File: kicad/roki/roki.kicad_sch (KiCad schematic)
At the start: 130 parts, among them SW1 RotaryEncoder_Switch, SW2 SW_SPDT, SW3 RotaryEncoder_Switch, SW4 SW_SPDT, U1 Nice_Nano_V2, U4 Nice_Nano_V2

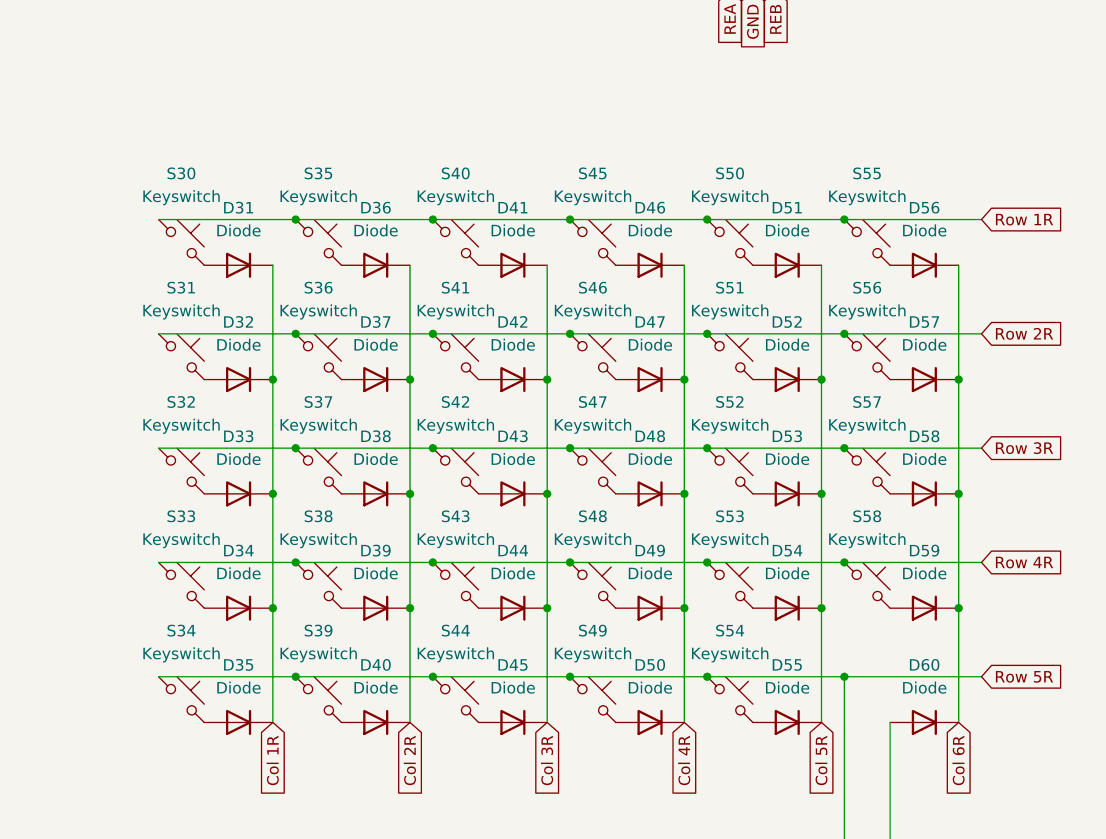
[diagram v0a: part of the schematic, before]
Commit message: feat(kicad): update pcb
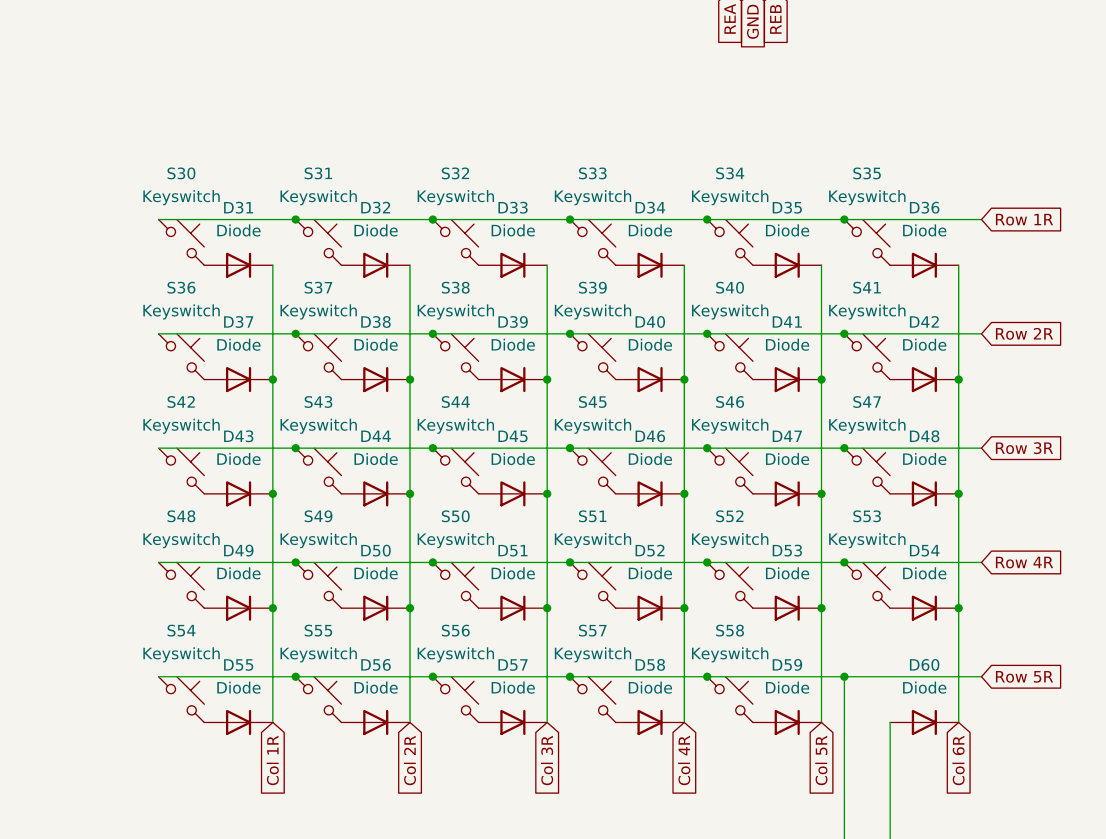
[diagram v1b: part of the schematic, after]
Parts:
- renumbered D36 to D32, D41 to D33, D46 to D34, D51 to D35, D56 to D36, D32 to D37, D37 to D38, D42 to D39, D47 to D40, D52 to D41, D57 to D42, D33 to D43, D38 to D44, D43 to D45, D48 to D46, D53 to D47, D58 to D48, D34 to D49, D39 to D50, D44 to D51, D49 to D52, D54 to D53, D59 to D54, D35 to D55, D40 to D56, D45 to D57, D50 to D58, D55 to D59, S35 to S31, S40 to S32, S45 to S33, S50 to S34, S55 to S35, S31 to S36, S36 to S37, S41 to S38, S46 to S39, S51 to S40, S56 to S41, S32 to S42, S37 to S43, S42 to S44, S47 to S45, S52 to S46, S57 to S47, S33 to S48, S38 to S49, S43 to S50, S48 to S51, S53 to S52, S58 to S53, S34 to S54, S39 to S55, S44 to S56, S49 to S57, S54 to S58
